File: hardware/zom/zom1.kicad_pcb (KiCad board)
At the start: 2 copper layers, 2 parts, among them U1 ESP32-WROOM, U2 RFM95HW

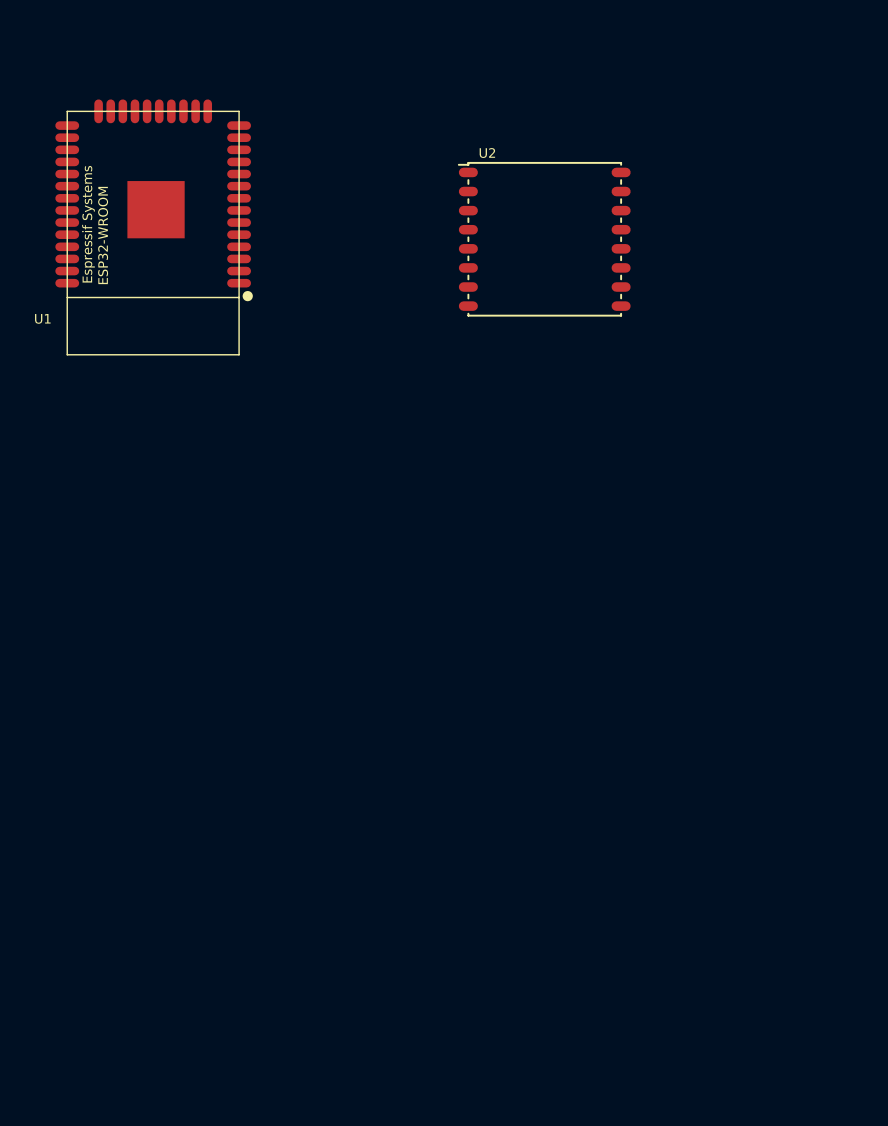
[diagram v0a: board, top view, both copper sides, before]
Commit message: update
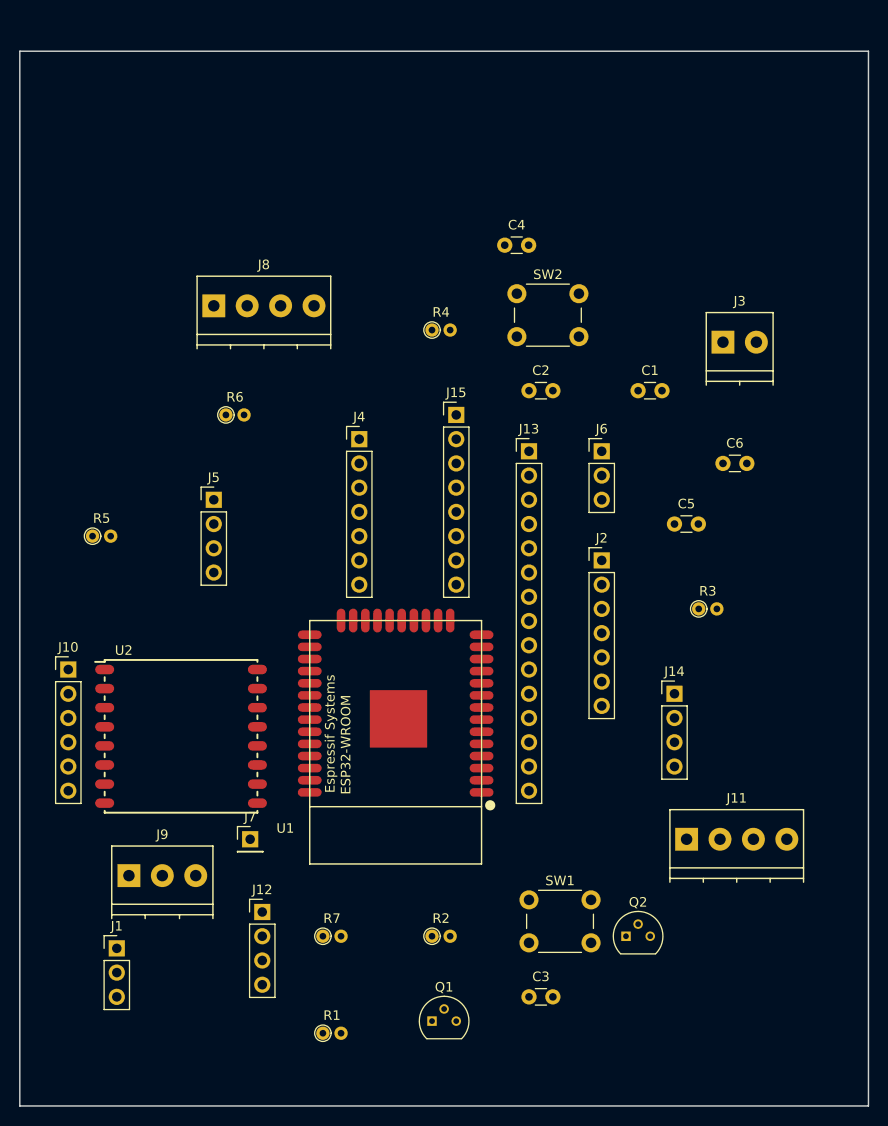
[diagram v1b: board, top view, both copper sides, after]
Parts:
- added C1: 10 uF, Capacitors_THT:C_Disc_D3.0mm_W1.6mm_P2.50mm, F.Cu at (86.4, 53.3)
- added C2: 22 uF, Capacitors_THT:C_Disc_D3.0mm_W1.6mm_P2.50mm, F.Cu at (74.9, 53.3)
- added C3: C, Capacitors_THT:C_Disc_D3.0mm_W1.6mm_P2.50mm, F.Cu at (74.9, 116.8)
- added C4: C, Capacitors_THT:C_Disc_D3.0mm_W1.6mm_P2.50mm, F.Cu at (72.4, 38.1)
- added C5: 10 uF, Capacitors_THT:C_Disc_D3.0mm_W1.6mm_P2.50mm, F.Cu at (90.2, 67.3)
- added C6: 22 uF, Capacitors_THT:C_Disc_D3.0mm_W1.6mm_P2.50mm, F.Cu at (95.2, 61.0)
- added J1: Conn_01x03, Socket_Strips:Socket_Strip_Straight_1x03_Pitch2.54mm, F.Cu at (31.8, 111.8)
- added J10: Conn_01x06, Pin_Headers:Pin_Header_Straight_1x06_Pitch2.54mm, F.Cu at (26.7, 82.5)
- added J11: Conn_01x04, TerminalBlocks_Phoenix:TerminalBlock_Phoenix_PT-3.5mm_4pol, F.Cu at (91.4, 100.3)
- added J12: Conn_01x04, Pin_Headers:Pin_Header_Straight_1x04_Pitch2.54mm, F.Cu at (47.0, 108.0)
- added J13: Conn_01x15, Socket_Strips:Socket_Strip_Straight_1x15_Pitch2.54mm, F.Cu at (74.9, 59.7)
- added J14: Conn_01x04, Pin_Headers:Pin_Header_Straight_1x04_Pitch2.54mm, F.Cu at (90.2, 85.1)
- added J15: Conn_01x08, Socket_Strips:Socket_Strip_Straight_1x08_Pitch2.54mm, F.Cu at (67.3, 55.9)
- added J2: Conn_01x07, Pin_Headers:Pin_Header_Straight_1x07_Pitch2.54mm, F.Cu at (82.5, 71.1)
- added J3: Conn_01x02, TerminalBlocks_Phoenix:TerminalBlock_Phoenix_PT-3.5mm_2pol, F.Cu at (95.2, 48.3)
- added J4: Conn_01x07, Pin_Headers:Pin_Header_Straight_1x07_Pitch2.54mm, F.Cu at (57.1, 58.4)
- added J5: Conn_01x04, Pin_Headers:Pin_Header_Straight_1x04_Pitch2.54mm, F.Cu at (41.9, 64.8)
- added J6: Conn_01x03, Pin_Headers:Pin_Header_Straight_1x03_Pitch2.54mm, F.Cu at (82.5, 59.7)
- added J7: Conn_01x01, Pin_Headers:Pin_Header_Straight_1x01_Pitch2.54mm, F.Cu at (45.7, 100.3)
- added J8: Conn_01x04, TerminalBlocks_Phoenix:TerminalBlock_Phoenix_PT-3.5mm_4pol, F.Cu at (41.9, 44.5)
- added J9: Conn_01x03, TerminalBlocks_Phoenix:TerminalBlock_Phoenix_PT-3.5mm_3pol, F.Cu at (33.0, 104.1)
- added Q1: Q_NPN_CBE, TO_SOT_Packages_THT:TO-92_Molded_Narrow, F.Cu at (64.8, 119.4)
- added Q2: Q_NPN_CBE, TO_SOT_Packages_THT:TO-92_Molded_Narrow, F.Cu at (85.1, 110.5)
- added R1: 10K, Resistors_THT:R_Axial_DIN0204_L3.6mm_D1.6mm_P1.90mm_Vertical, F.Cu at (53.3, 120.7)
- added R2: R, Resistors_THT:R_Axial_DIN0204_L3.6mm_D1.6mm_P1.90mm_Vertical, F.Cu at (64.8, 110.5)
- added R3: R, Resistors_THT:R_Axial_DIN0204_L3.6mm_D1.6mm_P1.90mm_Vertical, F.Cu at (92.7, 76.2)
- added R4: 10K, Resistors_THT:R_Axial_DIN0204_L3.6mm_D1.6mm_P1.90mm_Vertical, F.Cu at (64.8, 47.0)
- added R5: R, Resistors_THT:R_Axial_DIN0204_L3.6mm_D1.6mm_P1.90mm_Vertical, F.Cu at (29.2, 68.6)
- added R6: R, Resistors_THT:R_Axial_DIN0204_L3.6mm_D1.6mm_P1.90mm_Vertical, F.Cu at (43.2, 55.9)
- added R7: R, Resistors_THT:R_Axial_DIN0204_L3.6mm_D1.6mm_P1.90mm_Vertical, F.Cu at (53.3, 110.5)
- added SW1: SW_Push, Buttons_Switches_THT:SW_PUSH_6mm, F.Cu at (74.9, 106.7)
- added SW2: SW_Push, Buttons_Switches_THT:SW_PUSH_6mm, F.Cu at (73.7, 43.2)
- moved U2 64.5 mm to (30.5, 82.5)
- moved U1 59.1 mm to (61.0, 90.2)
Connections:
- U1 pad 1: Net-(U1-Pad1) -> GND
- U1 pad 10: Net-(U1-Pad10) -> 25
- U1 pad 11: Net-(U1-Pad11) -> 26
- U1 pad 12: Net-(U1-Pad12) -> 27/SAT_SLEEP
- U1 pad 13: Net-(U1-Pad13) -> 14
- U1 pad 14: Net-(U1-Pad14) -> 12
- U1 pad 15: Net-(U1-Pad15) -> GND
- U1 pad 16: Net-(U1-Pad16) -> 13
- U1 pad 17: Net-(U1-Pad17) -> (no net)
- U1 pad 18: Net-(U1-Pad18) -> (no net)
- U1 pad 19: Net-(U1-Pad19) -> (no net)
- U1 pad 2: Net-(U1-Pad2) -> 22
- U1 pad 20: Net-(U1-Pad20) -> (no net)
- U1 pad 21: Net-(U1-Pad21) -> (no net)
- U1 pad 22: Net-(U1-Pad22) -> (no net)
- U1 pad 23: Net-(U1-Pad23) -> (no net)
- U1 pad 24: Net-(U1-Pad24) -> 2
- U1 pad 25: Net-(U1-Pad25) -> 0
- U1 pad 26: Net-(U1-Pad26) -> SDA
- U1 pad 27: Net-(U1-Pad27) -> SCL
- U1 pad 28: Net-(U1-Pad28) -> 17
- U1 pad 29: Net-(U1-Pad29) -> 5
- U1 pad 3: Net-(U1-Pad3) -> RESET
- U1 pad 30: Net-(U1-Pad30) -> 18
- U1 pad 31: Net-(U1-Pad31) -> 19
- U1 pad 32: Net-(U1-Pad32) -> (no net)
- U1 pad 33: Net-(U1-Pad33) -> 21
- U1 pad 34: Net-(U1-Pad34) -> (no net)
- U1 pad 35: Net-(U1-Pad35) -> (no net)
- U1 pad 36: Net-(U1-Pad36) -> 22
- U1 pad 37: Net-(U1-Pad37) -> 23
- U1 pad 38: Net-(U1-Pad38) -> GND
- U1 pad 39: Net-(U1-Pad39) -> GND
- U1 pad 4: Net-(U1-Pad4) -> (no net)
- U1 pad 5: Net-(U1-Pad5) -> (no net)
- U1 pad 6: Net-(U1-Pad6) -> 34/RX1
- U1 pad 7: Net-(U1-Pad7) -> 35/RX2
- U1 pad 8: Net-(U1-Pad8) -> 32/TX1
- U1 pad 9: Net-(U1-Pad9) -> 33/TX2
- U2 pad 1: Net-(U2-Pad1) -> GND
- U2 pad 10: Net-(U2-Pad10) -> GND
- U2 pad 13: Net-(U2-Pad13) -> 22
- U2 pad 2: Net-(U2-Pad2) -> 19
- U2 pad 3: Net-(U2-Pad3) -> 18
- U2 pad 4: Net-(U2-Pad4) -> 5
- U2 pad 5: Net-(U2-Pad5) -> 12
- U2 pad 6: Net-(U2-Pad6) -> (no net)
- U2 pad 8: Net-(U2-Pad8) -> GND
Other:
- board outline added: 88.9 x 110.5 mm

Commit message: update
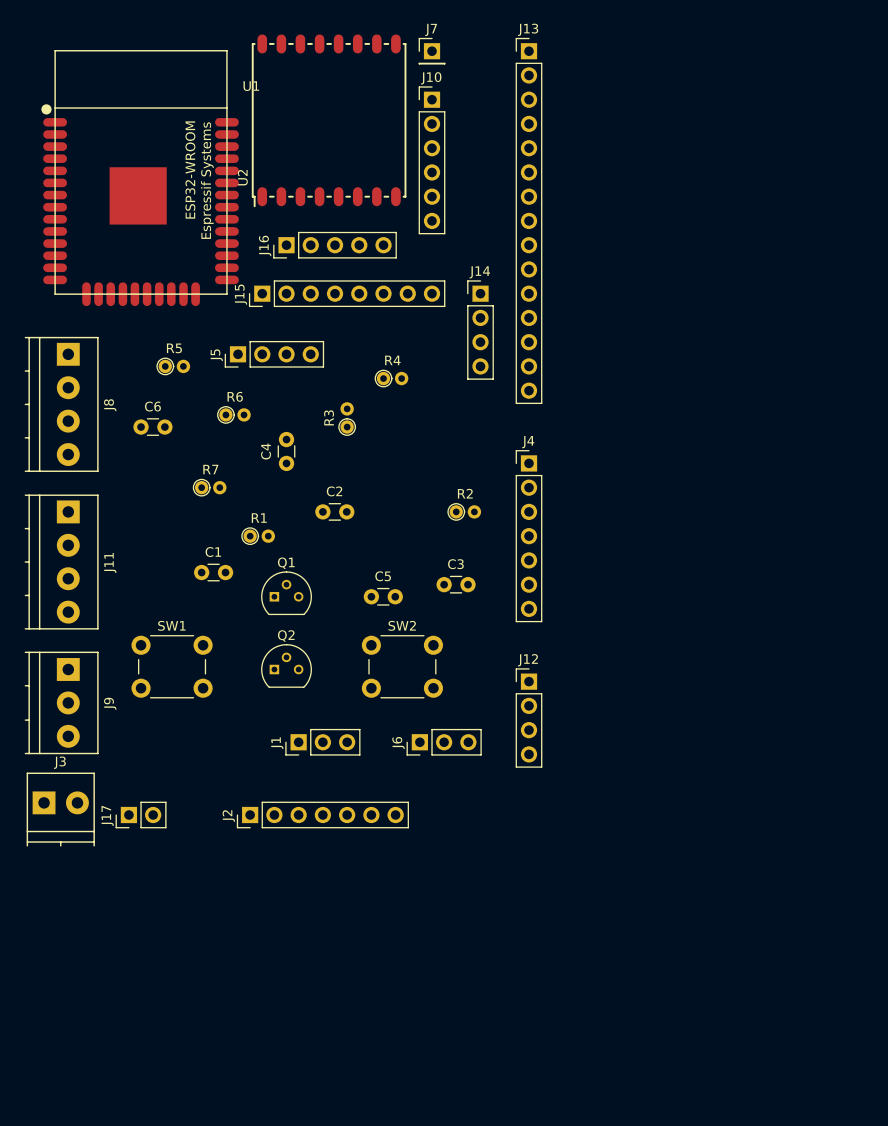
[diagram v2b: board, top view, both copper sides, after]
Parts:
- added J16: LBO, Pin_Headers:Pin_Header_Straight_1x05_Pitch2.54mm, F.Cu at (49.5, 38.1)
- added J17: VIN2, Pin_Headers:Pin_Header_Straight_1x02_Pitch2.54mm, F.Cu at (33.0, 97.8)
- J1: value Conn_01x03 -> REG:3V3
- J10: value Conn_01x06 -> LBD
- J11: value Conn_01x04 -> UART
- J12: value Conn_01x04 -> dht22
- J13: value Conn_01x15 -> 9602
- J14: value Conn_01x04 -> satx
- J15: value Conn_01x08 -> MISC
- J2: value Conn_01x07 -> prog
- J3: value Conn_01x02 -> VINS
- J4: value Conn_01x07 -> sdcard
- J5: value Conn_01x04 -> oled
- J6: value Conn_01x03 -> REG:5V
- J7: value Conn_01x01 -> ANT
- J8: value Conn_01x04 -> i2c
- J9: value Conn_01x03 -> 1wire
- moved J3 85.9 mm to (24.1, 96.5)
- moved J7 84.7 mm to (64.8, 17.8)
- moved J11 73.3 mm to (26.7, 66.0), turned to 270 degrees
- moved J10 70.8 mm to (64.8, 22.9)
- moved U1 65.4 mm to (34.3, 30.5), turned to 180 degrees
- moved C6 61.1 mm to (34.3, 57.1)
- moved R1 52.6 mm to (45.7, 68.6)
- moved U2 52.2 mm to (47.0, 33.0), turned to 90 degrees
- moved C1 49.5 mm to (40.6, 72.4)
- moved R7 48.7 mm to (40.6, 63.5)
- moved SW1 48.6 mm to (34.3, 80.0)
- moved Q1 47.4 mm to (48.3, 74.9)
- moved J14 46.6 mm to (69.8, 43.2)
- moved Q2 46.2 mm to (48.3, 82.5)
- moved J2 45.5 mm to (45.7, 97.8), turned to 90 degrees
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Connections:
- U1 pad 23: (no net) -> 15
- U2 pad 6: (no net) -> 15
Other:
- board outline removed
